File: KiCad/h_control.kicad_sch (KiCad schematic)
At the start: 14 parts, among them J4 Conn_02x05_Odd_Even, SW1 SW_Push, U9 ATSAMD21E15B-M

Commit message: Use 0603 resistors and capacitors
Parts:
- C4, C5, C6, C7: footprint Capacitor_SMD:C_0805_2012Metric -> Capacitor_SMD:C_0603_1608Metric
- R1, R19, R2, R3: footprint Resistor_SMD:R_0805_2012Metric -> Resistor_SMD:R_0603_1608Metric
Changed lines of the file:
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@@
     (property "Reference" "R2" (id 0) (at 118.11 69.85 90))
     (property "Value" "220" (id 1) (at 125.73 69.85 90))
-    (property "Footprint" "Resistor_SMD:R_0805_2012Metric" (id 2) (at 121.92 68.58 0)
+    (property "Footprint" "Resistor_SMD:R_0603_1608Metric" (id 2) (at 121.92 68.58 0)
       (effects (font (size 1.27 1.27)) hide)
     )
@@
     (property "Reference" "R1" (id 0) (at 118.11 105.41 90))
     (property "Value" "220" (id 1) (at 125.73 105.41 90))
-    (property "Footprint" "Resistor_SMD:R_0805_2012Metric" (id 2) (at 121.92 104.14 0)
+    (property "Footprint" "Resistor_SMD:R_0603_1608Metric" (id 2) (at 121.92 104.14 0)
       (effects (font (size 1.27 1.27)) hide)
     )
@@
       (effects (font (size 1.27 1.27)) (justify left))
     )
-    (property "Footprint" "Capacitor_SMD:C_0805_2012Metric" (id 2) (at 121.92 46.99 0)
+    (property "Footprint" "Capacitor_SMD:C_0603_1608Metric" (id 2) (at 121.92 46.99 0)
       (effects (font (size 1.27 1.27)) hide)
     )
@@
       (effects (font (size 1.27 1.27)) (justify left))
     )
-    (property "Footprint" "Capacitor_SMD:C_0805_2012Metric" (id 2) (at 133.35 46.99 0)
+    (property "Footprint" "Capacitor_SMD:C_0603_1608Metric" (id 2) (at 133.35 46.99 0)
       (effects (font (size 1.27 1.27)) hide)
     )
@@
     (property "Reference" "R19" (id 0) (at 118.11 130.81 90))
     (property "Value" "1k" (id 1) (at 118.11 135.89 90))
-    (property "Footprint" "Resistor_SMD:R_0805_2012Metric" (id 2) (at 118.11 133.35 0)
+    (property "Footprint" "Resistor_SMD:R_0603_1608Metric" (id 2) (at 118.11 133.35 0)
       (effects (font (size 1.27 1.27)) hide)
     )
@@
     (property "Reference" "R3" (id 0) (at 118.11 100.33 90))
     (property "Value" "220" (id 1) (at 125.73 100.33 90))
-    (property "Footprint" "Resistor_SMD:R_0805_2012Metric" (id 2) (at 121.92 101.6 0)
+    (property "Footprint" "Resistor_SMD:R_0603_1608Metric" (id 2) (at 121.92 101.6 0)
       (effects (font (size 1.27 1.27)) hide)
     )
@@
       (effects (font (size 1.27 1.27)) (justify left))
     )
-    (property "Footprint" "Capacitor_SMD:C_0805_2012Metric" (id 2) (at 189.23 46.99 0)
+    (property "Footprint" "Capacitor_SMD:C_0603_1608Metric" (id 2) (at 189.23 46.99 0)
       (effects (font (size 1.27 1.27)) hide)
     )
@@
       (effects (font (size 1.27 1.27)) (justify left))
     )
-    (property "Footprint" "Capacitor_SMD:C_0805_2012Metric" (id 2) (at 177.8 46.99 0)
-      (effects (font (size 1.27 1.27)) hide)
-    )
+    (property "Footprint" "Capacitor_SMD:C_0603_1608Metric" (id 2) (at 177.8 46.99 0)
+      (effects (font (size 1.27 1.27)) hide)
+    )

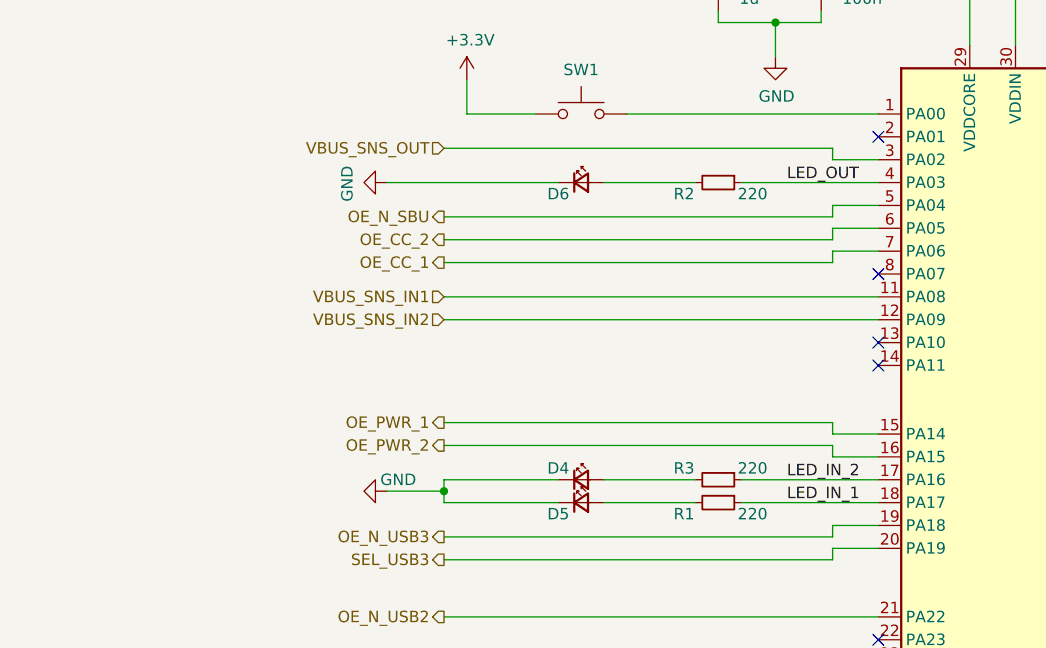
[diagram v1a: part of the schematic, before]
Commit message: CC detect trigger + inner layer routing
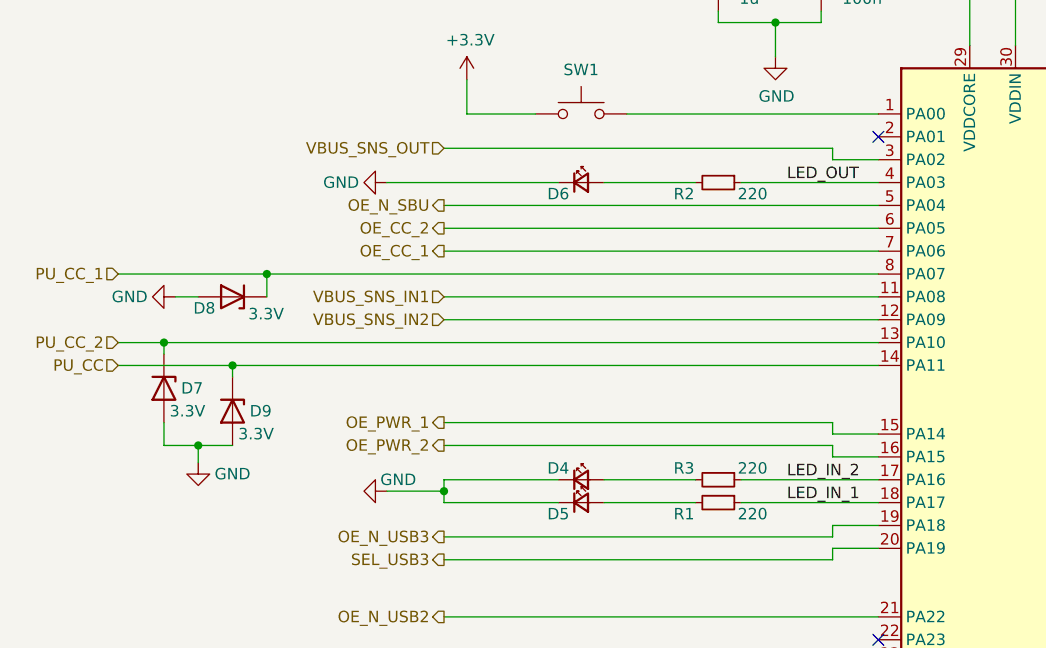
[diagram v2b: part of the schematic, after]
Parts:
- added D7, D8, D9: 3.3V, Diode_SMD:D_SOD-523, symbol Diode:BZV55B3V3
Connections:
- net GND: now also D7.2 (A), D8.2 (A), D9.2 (A)
- net PU_CC_2: now reaches U9.13 (PA10)
- net PU_CC_2: now also D7.1 (K)
- net PU_CC: now reaches U9.14 (PA11)
- net PU_CC: now also D9.1 (K)
- net PU_CC_1: now reaches U9.8 (PA07)
- net PU_CC_1: now also D8.1 (K)
- no-connect marks 8 -> 5
